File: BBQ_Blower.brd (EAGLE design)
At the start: 95.9 x 84.8 mm, 31 parts, among them IC1 MAX31855RASA+, IC2 MAX31855RASA+, IC3 MAX31855RASA+, J1 1X2-3.5MM, J10 1X2-3.5MM, J11 1X2-3.5MM, J2 1X2-3.5MM, J3 PCC-SMP-K-100-R-ROHS, J4 PCC-SMP-K-100-R-ROHS, J5 1X2-3.5MM, J6 1X2-3.5MM, J7 1X2-3.5MM, J9 1X2-3.5MM, K1 SRD-12VDC-SL-C, K2 SRD-12VDC-SL-C, Q1 BUZ10, Q2 BUZ10, T1 2N3904, T2 2N3904, U1 113990105

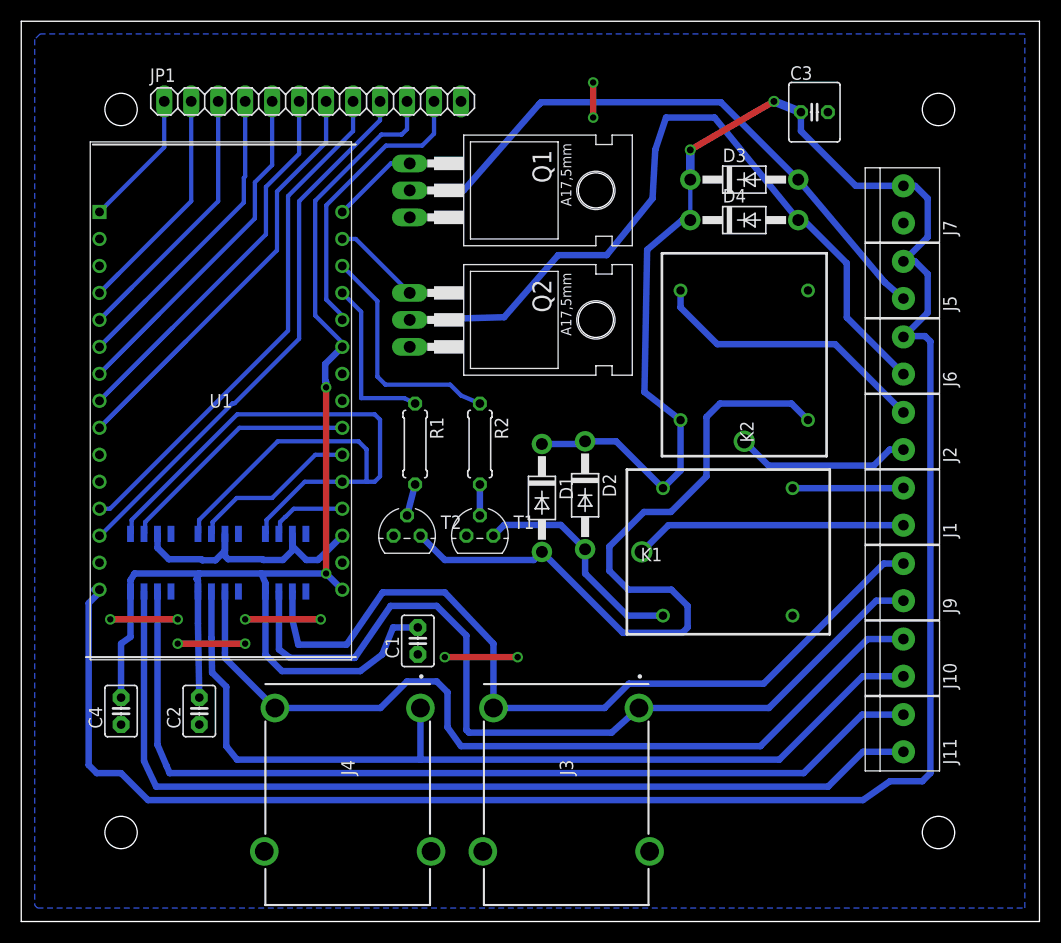
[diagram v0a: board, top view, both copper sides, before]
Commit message: initial
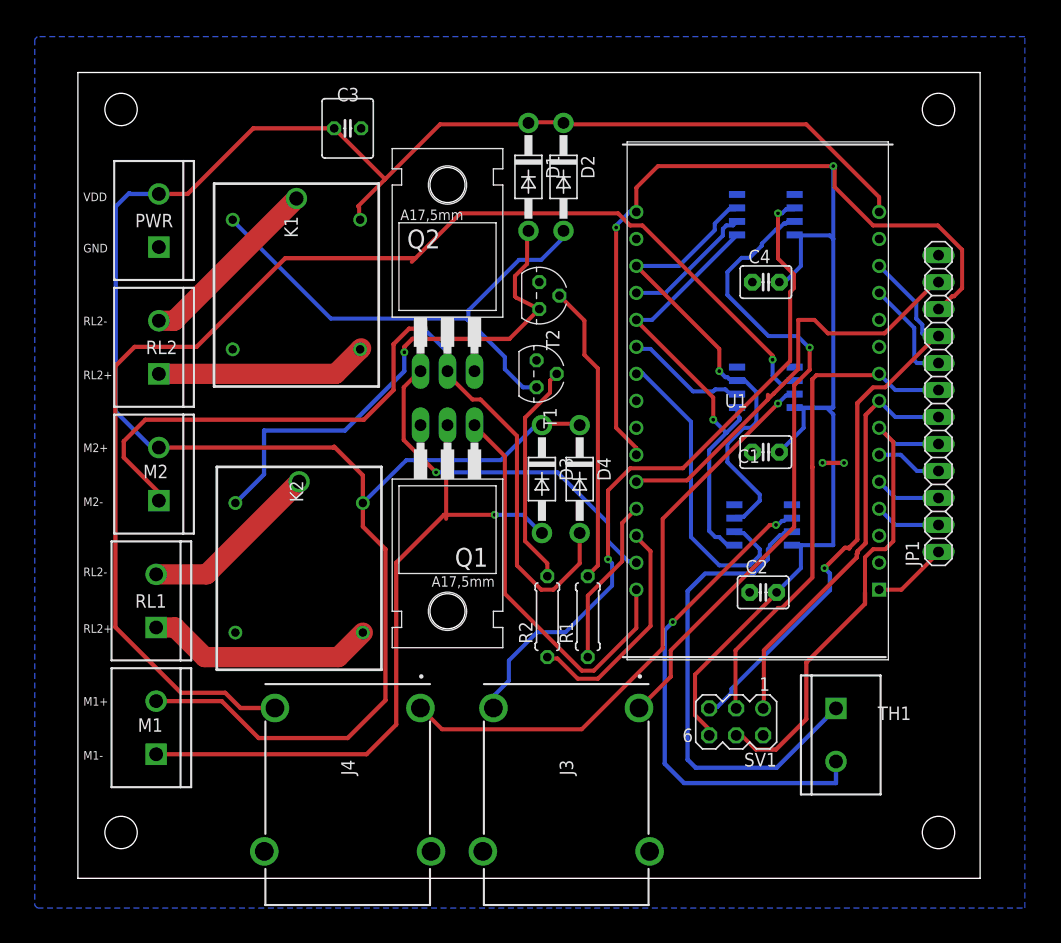
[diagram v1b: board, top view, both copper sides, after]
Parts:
- removed J1, J10, J11, J2, J5, J6, J7, J9: 1X2-3.5MM, adafruit:1X2-3.5MM
- added M1, M2, PWR, RL1, RL2, TH1: (no value), SparkFun-Connectors:SCREWTERMINAL-5MM-2
- added SV1: (no value), con-lstb:MA03-2
- moved C4 72.9 mm to (70.1, 60.2), turned to 0 degrees
- moved JP1 65.4 mm to (86.4, 48.8), turned to 90 degrees
- moved IC3 57.8 mm to (69.8, 37.3), turned to 0 degrees
- moved IC1 55.8 mm to (70.1, 66.5), turned to 0 degrees
- moved C2 54.2 mm to (69.8, 31.0), turned to 0 degrees
- moved IC2 54.1 mm to (70.1, 50.3), turned to 0 degrees
- moved U1 50.5 mm to (69.3, 49.0), turned to 180 degrees
- moved K1 46.5 mm to (25.9, 68.1), turned to 270 degrees
- moved C3 44.0 mm to (30.7, 74.7)
- moved K2 42.1 mm to (26.2, 41.4), turned to 270 degrees
- moved C1 37.3 mm to (70.1, 44.2), turned to 0 degrees
- moved D3 34.0 mm to (49.0, 41.7), turned to 270 degrees
- moved D1 30.3 mm to (47.8, 70.1)
- moved D2 30.0 mm to (51.1, 70.1)
- moved D4 28.9 mm to (52.6, 41.7), turned to 270 degrees
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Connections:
- removed net CMD: JP1.5, U1.7
- removed net D0: JP1.6, U1.8
- new net MISO: JP1.6, SV1.1, U1.8
- new net MOSI: JP1.5, SV1.4, U1.7
- net 3V3: now also SV1.6
- net BLOWER1: now also M2.1; no longer J6.1
- net BLOWER2: now also M1.1; no longer J5.1
- net CLK: now also SV1.3
- net GND: now also PWR.1, SV1.2; no longer J7.1
- net RELAY1(+): now also RL2.1; no longer J1.2
- net RELAY1(-): now also RL2.2; no longer J1.1
- net RELAY2(+): now also RL1.1; no longer J2.2
- net RELAY2(-): now also RL1.2; no longer J2.1
- net RST: now also SV1.5
- net T1+: no longer J9.1
- net T1-: no longer J9.2
- net T2+: no longer J10.1
- net T2-: no longer J10.2
- net T3+: now also TH1.1; no longer J11.1
- net T3-: now also TH1.2; no longer J11.2
- net VDD: now also M1.2, M2.2, PWR.2; no longer J5.2, J6.2, J7.2
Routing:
- net MOSI: track 0.00 -> 46.6 mm
- net D0: track 45.7 -> 0.00 mm
- net T3+: track 90.3 -> 45.3 mm
- net T3-: track 88.7 -> 47.8 mm, vias 0 -> 2
- net CMD: track 40.3 -> 0.00 mm
- net MISO: track 0.00 -> 39.7 mm
- net T2-: track 81.9 -> 121.3 mm, vias 0 -> 1
- net EN: track 48.8 -> 10.1 mm
- net VDD: track 237.2 -> 203.9 mm, vias 2 -> 0
- net 3V3: track 120.4 -> 153.4 mm
- net T2+: track 87.6 -> 56.4 mm, vias 0 -> 1
- net BLOWER_1: track 8.24 -> 37.7 mm
- net SCK: track 71.7 -> 42.8 mm, vias 0 -> 1
- net D1: track 34.9 -> 6.22 mm
- net GND: track 30.0 -> 2.03 mm, vias 10 -> 2
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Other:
- board size 95.9 x 84.8 mm -> 84.9 x 75.9 mm
- board text added: "Board: BBQ Controller Author: Cody Fischer Date: November 2018 Rev: 1.0"
- board text added: "GND"
- board text added: "M1+"
- board text added: "M1-"
- board text added: "M2+"
- board text added: "M2-"
- board text added: "RL2+"
- board text added: "RL2-"
- board text added: "VDD"
